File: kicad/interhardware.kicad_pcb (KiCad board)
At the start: 2 copper layers, 72.2 x 56.2 mm, 65 parts, among them J1 RJE0166002, J2 USB_C_Receptacle_USB2.0_16P, Q1 MMBTA42, Q2 MMBTA92, Q3 MMBTA42, Q4 MMBTA06, Q5 MMBTA06, SW1 B3U-1000P, U3 ESP32-C3-WROOM-02, U4 TPS62162DSG

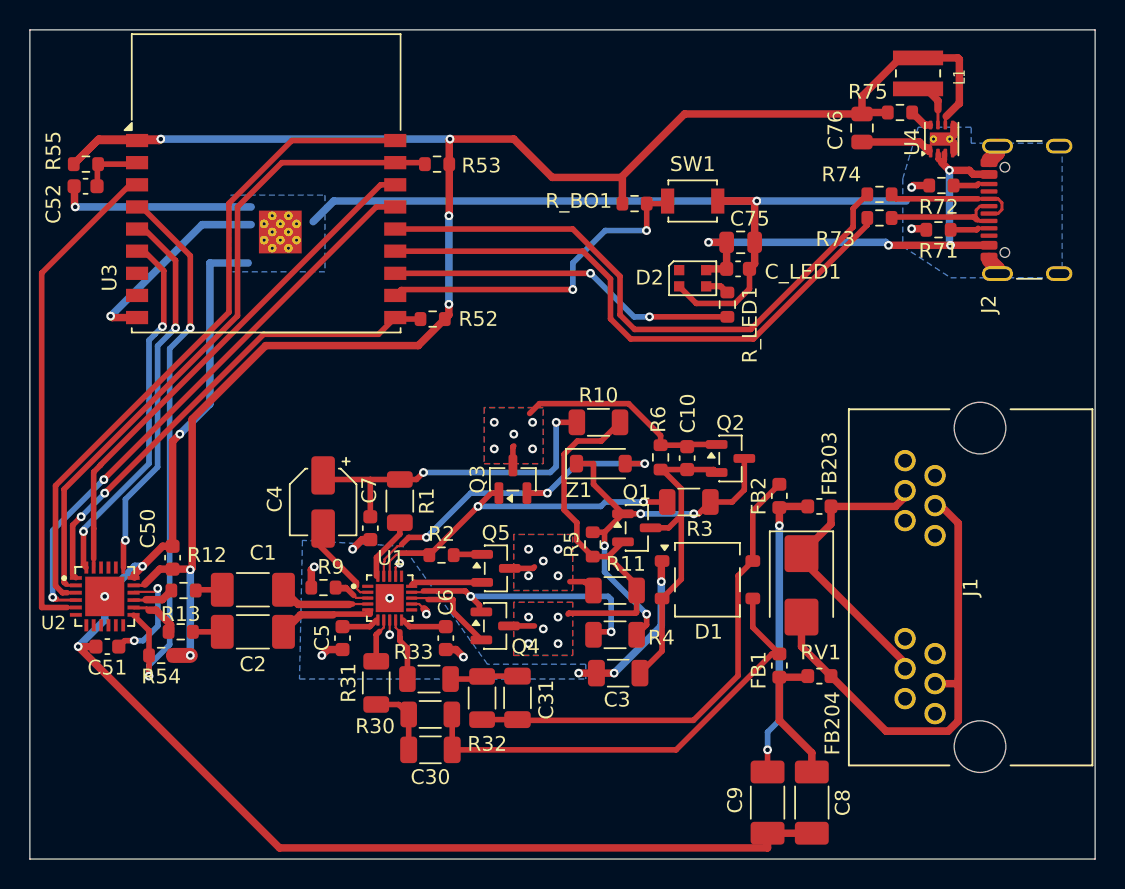
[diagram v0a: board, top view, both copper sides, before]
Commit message: edit pra deixar 100%
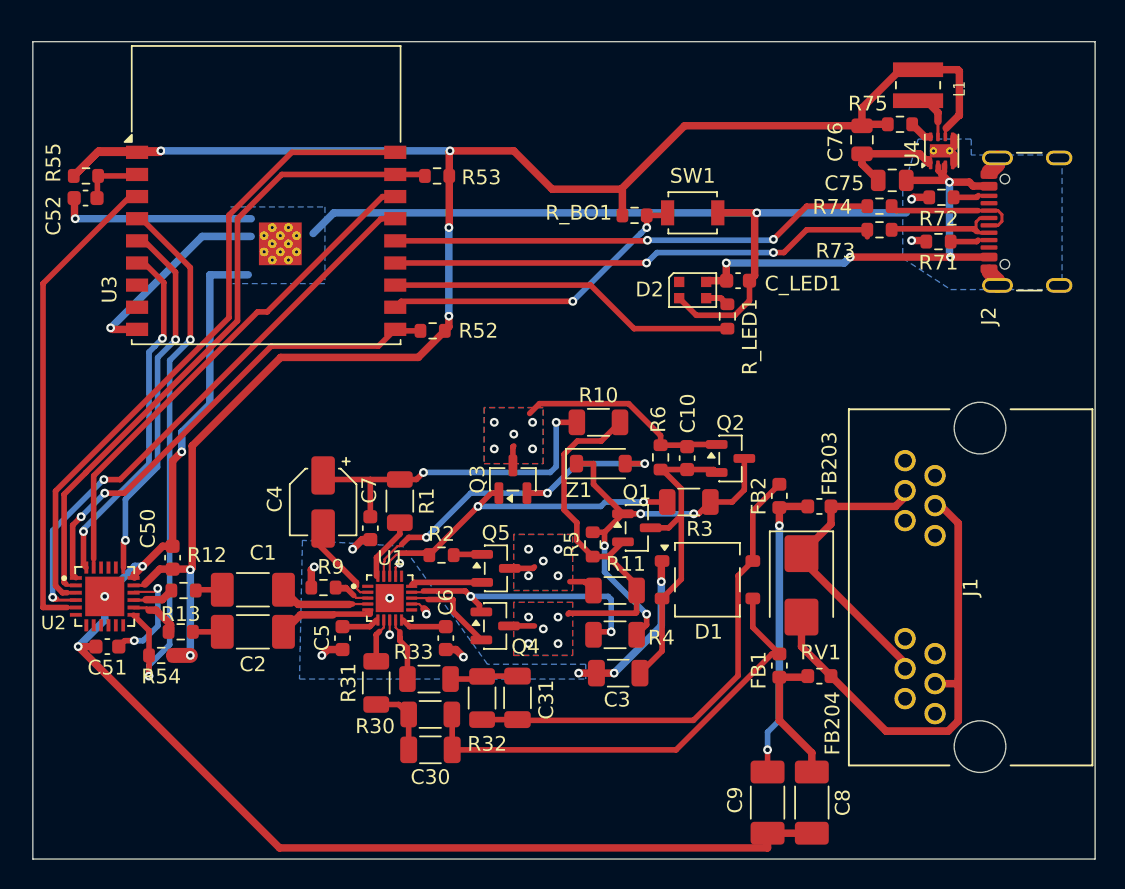
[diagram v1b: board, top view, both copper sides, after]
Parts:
- moved C75 11.1 mm to (245.7, 92.4), turned to 180 degrees
- moved C76 0.80 mm to (243.6, 89.7)
- moved R74 0.80 mm to (244.8, 94.2)
- moved R_BO1 0.80 mm to (228.2, 94.8)
- moved U4 0.80 mm to (249.0, 90.4)
- moved C52 0.80 mm to (191.0, 93.6)
- moved C_LED1 0.80 mm to (235.2, 99.2)
- moved D2 0.80 mm to (232.1, 99.8)
- moved J2 0.80 mm to (255.9, 95.2)
- moved L1 0.80 mm to (247.4, 86.0)
- moved R52 0.80 mm to (214.5, 102.6)
- moved R53 0.80 mm to (214.8, 92.1)
- moved R55 0.80 mm to (191.0, 92.1)
- moved R71 0.80 mm to (248.8, 96.5)
- moved R72 0.80 mm to (249.0, 93.5)
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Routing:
- net Net-(U3-IO19): track 40.9 -> 33.0 mm, vias 0 -> 2
- net Net-(U3-IO18): track 39.7 -> 33.4 mm, vias 0 -> 2
- net Net-(U3-IO20/RXD): track 23.2 -> 21.6 mm
- net GND: track 186.8 -> 188.2 mm
- net +3.3V: track 134.5 -> 133.1 mm
- net /DRX: track 33.9 -> 33.0 mm
- net /SCLK: track 25.8 -> 25.0 mm
- net /PCLK: track 45.4 -> 44.6 mm
- net /SDI: track 24.8 -> 24.0 mm
- net /RESET: track 39.2 -> 38.4 mm
- net /FSYNC: track 45.1 -> 44.3 mm
- net Net-(U3-IO21/TXD): vias 2 -> 0
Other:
- board size 72.2 x 56.2 mm -> 72 x 55.4 mm
